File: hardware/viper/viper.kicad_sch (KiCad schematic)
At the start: 52 parts, among them J1 TYPE-C-31-M-12, Q1 2N7002, U1 ATmega32U4-A, U2 USBLC6-2SC6, Y1 16MHz

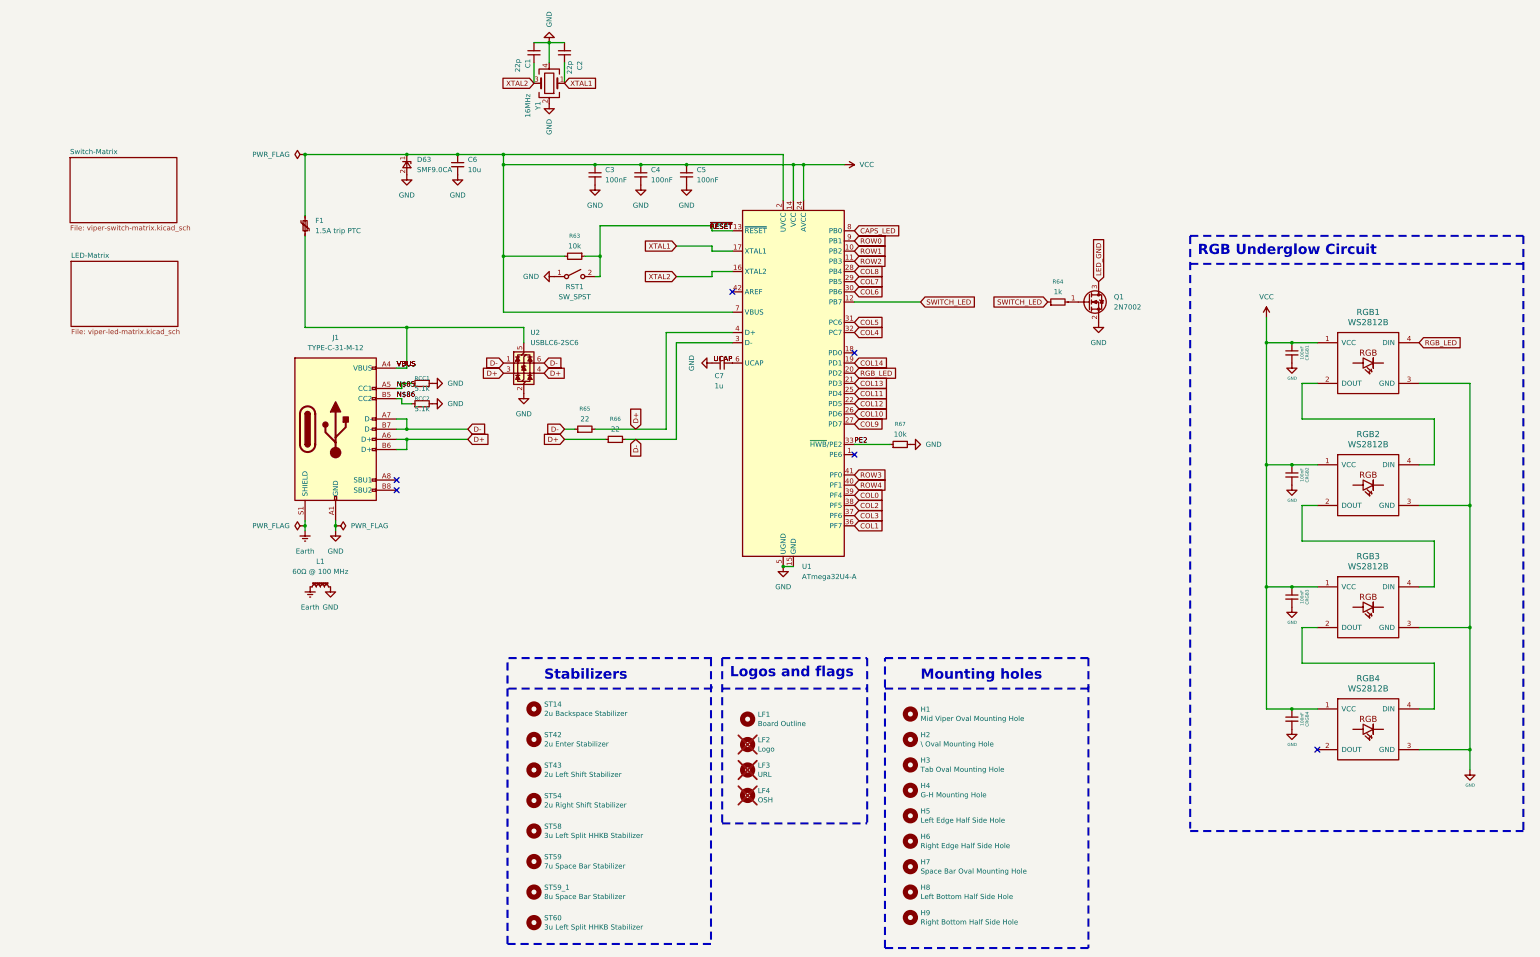
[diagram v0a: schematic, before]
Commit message: Improved schematic
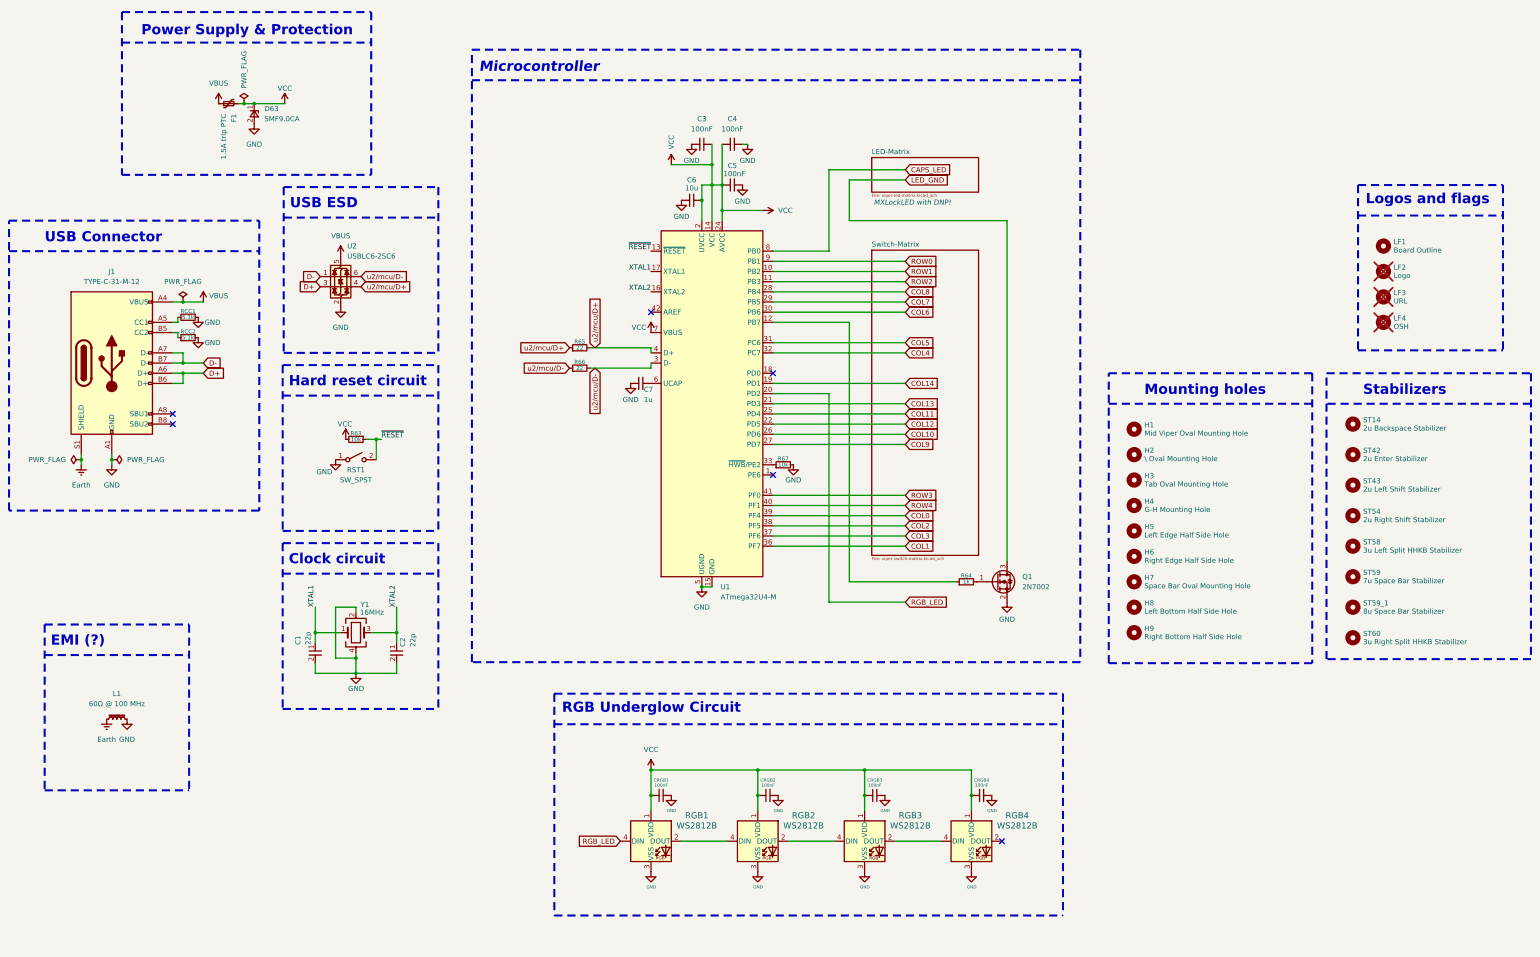
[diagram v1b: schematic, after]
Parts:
- H1: value Mid Viper Oval Mounting Hole -> ~
- H2: value \ Oval Mounting Hole -> ~
- H3: value Tab Oval Mounting Hole -> ~
- H4: value G-H Mounting Hole -> ~
- H5: value Left Edge Half Side Hole -> ~
- H6: value Right Edge Half Side Hole -> ~
- H7: value Space Bar Oval Mounting Hole -> ~
- H8: value Left Bottom Half Side Hole -> ~
- H9: value Right Bottom Half Side Hole -> ~
- LF1: value Board Outline -> ~
- LF2: value Logo -> ~
- LF3: value URL -> ~
- LF4: value OSH -> ~
- RGB1, RGB2, RGB3, RGB4: footprint locallib:LED_SMD3528-4P-WS2812B -> LED_SMD:LED_WS2812B_PLCC4_5.0x5.0mm_P3.2mm; symbol ws2812b:WS2812B -> LED:WS2812B
- ST14: value 2u Backspace Stabilizer -> ~
- ST42: value 2u Enter Stabilizer -> ~
- ST43: value 2u Left Shift Stabilizer -> ~
- ST54: value 2u Right Shift Stabilizer -> ~
- ST58, ST60: value 3u Left Split HHKB Stabilizer -> ~
- ST59: value 7u Space Bar Stabilizer -> ~
- ST59_1: value 8u Space Bar Stabilizer -> ~
- U1: value ATmega32U4-A -> ATmega32U4-M; symbol MCU_Microchip_ATmega:ATmega32U4-A -> MCU_Microchip_ATmega:ATmega32U4-M
- renumbered C2 to C1, C1 to C2, C4 to C3, C3 to C4
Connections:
- net D+: no longer R65.2, R66.1, U1.4 (D+), U2.4 (I/O2)
- net D-: no longer R65.1, R66.2, U1.3 (D-), U2.6 (I/O1)
- net GND: now also U1.45 (GND)
- net N$85: no longer names the net of J1.A5 (CC1), RCC1.2
- net N$86: no longer names the net of J1.B5 (CC2), RCC2.1
- net PE2: no longer names the net of R67.1, U1.33 (~{HWB}/PE2)
- net SWITCH_LED: no longer names the net of R64.1, U1.12 (PB7)
- net UCAP: no longer names the net of C7.1, U1.6 (UCAP)
- new net u2/mcu/D+: R65.1, R65.2, U1.4 (D+), U2.4 (I/O2)
- new net u2/mcu/D-: R66.1, R66.2, U1.3 (D-), U2.6 (I/O1)
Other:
- note added: "Clock circuit"
- note added: "EMI (?)"
- note added: "Hard reset circuit"
- note added: "Microcontroller"
- note added: "Power Supply & Protection"
- note added: "USB Connector"
- note added: "USB ESD"
- moved on the sheet: C3, C4, C5, C6, C7, CRGB1, CRGB2, CRGB3, CRGB4, D63, F1, H1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
